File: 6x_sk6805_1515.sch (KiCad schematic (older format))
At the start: 7 parts

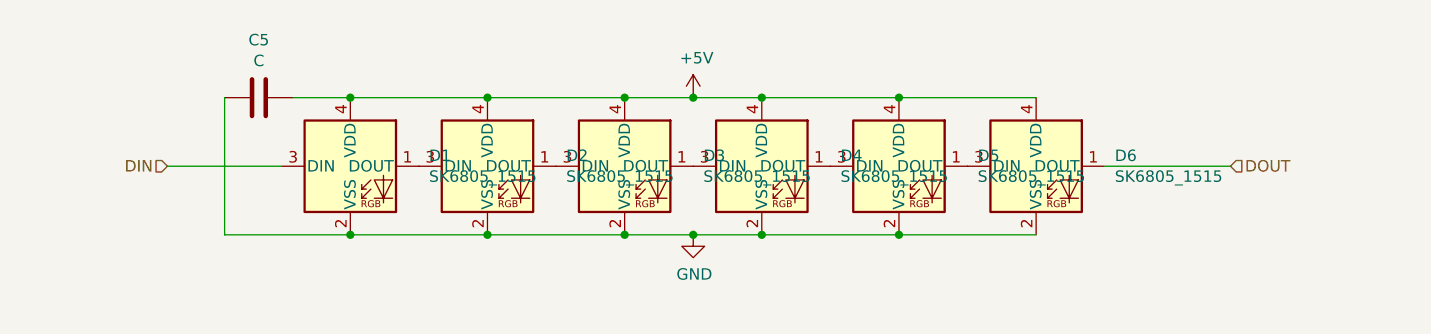
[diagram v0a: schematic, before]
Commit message: Some updates, not finished
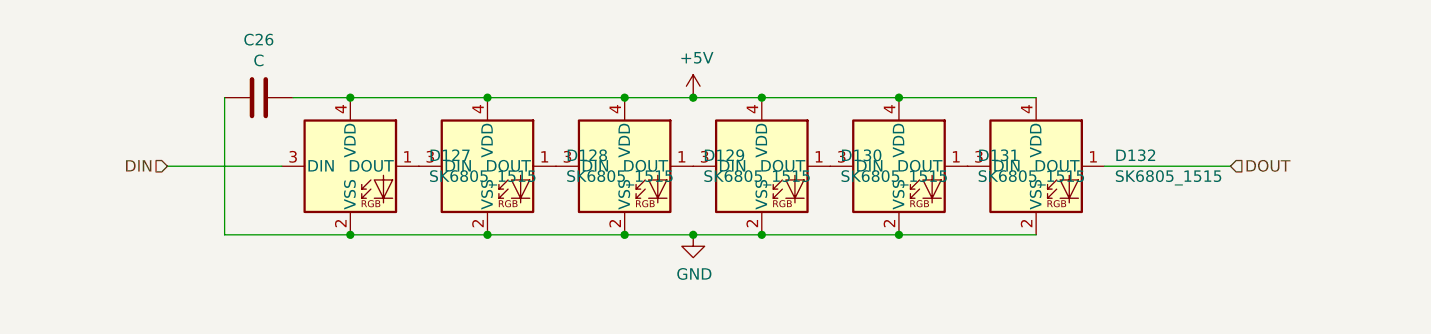
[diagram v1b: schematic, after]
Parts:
- renumbered C9 to C5, D25 to D1, D26 to D2, D27 to D3, D28 to D4, D29 to D5, D30 to D6

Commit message: Use atsamd21; do most layout
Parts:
- C21: renamed from C5; footprint Capacitor_SMD:C_0805_2012Metric -> Capacitor_SMD:C_0603_1608Metric
- D61: renamed from D1; symbol LED:SK6805_1515 -> WM_lib:SK6805_1515-LED
- D62: renamed from D2; symbol LED:SK6805_1515 -> WM_lib:SK6805_1515-LED
- D63: renamed from D3; symbol LED:SK6805_1515 -> WM_lib:SK6805_1515-LED
- D64: renamed from D4; symbol LED:SK6805_1515 -> WM_lib:SK6805_1515-LED
- D65: renamed from D5; symbol LED:SK6805_1515 -> WM_lib:SK6805_1515-LED
- D66: renamed from D6; symbol LED:SK6805_1515 -> WM_lib:SK6805_1515-LED
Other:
- moved on the sheet: C32, D128, D129, D130, D131, D132
